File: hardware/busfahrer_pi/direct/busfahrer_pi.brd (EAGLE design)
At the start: 39.4 x 37.8 mm, 21 parts, among them Q1 20 MHz, X1 MKDSN1,5/2-5,08

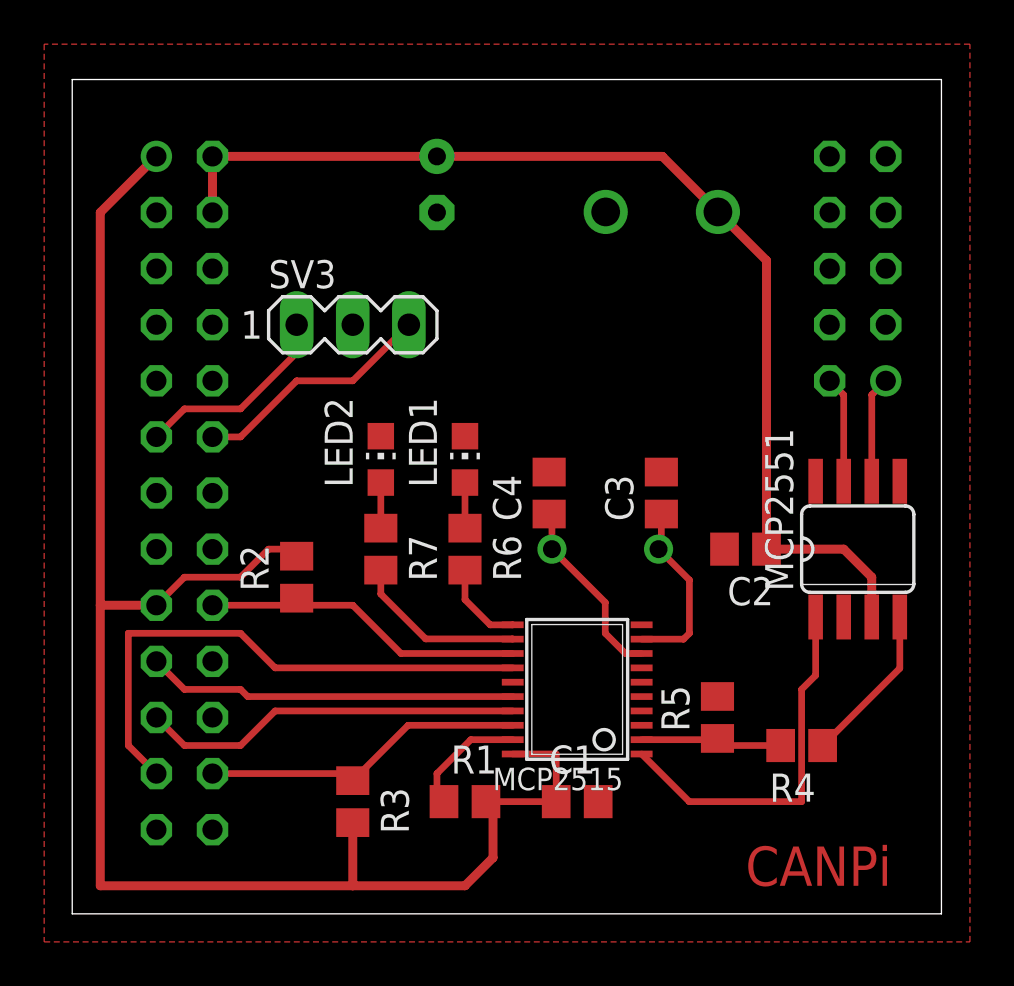
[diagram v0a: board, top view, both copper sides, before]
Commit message: some fixes
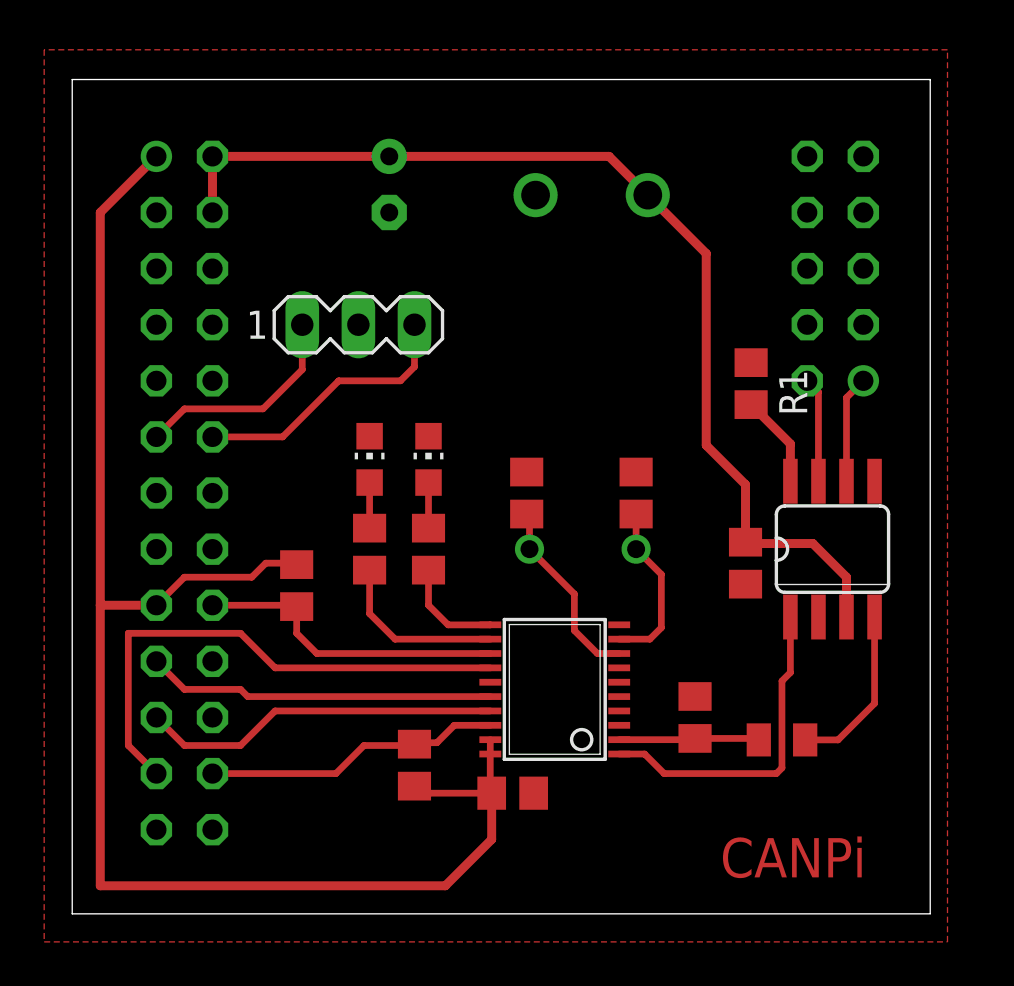
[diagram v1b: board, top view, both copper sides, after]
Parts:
- C3, C4: value 15p -> 22p
- R4: device rcl:R0805 -> rcl_patch:R0805
- R6, R7: value 220 -> 330
- moved R1 22.9 mm to (30.7, 24.0), turned to 270 degrees
- moved X1 3.27 mm to (23.5, 32.5)
- moved R3 3.25 mm to (15.5, 6.73)
- moved C1 2.95 mm to (19.9, 5.46)
- moved C5 2.16 mm to (14.4, 33.0)
- moved LED1 1.65 mm to (16.1, 20.6)
- moved R6 1.65 mm to (16.1, 16.5)
- moved C3 1.14 mm to (25.5, 19.1)
- moved MCP2551 1.14 mm to (34.4, 16.5)
- moved SV2 1.02 mm to (34.5, 29.2)
- moved R5 1.02 mm to (28.2, 8.89)
- moved C4 1.02 mm to (20.6, 19.1)
- moved MCP2515 1.02 mm to (21.8, 10.2)
- moved Q1 1.02 mm to (23.1, 16.5)
- moved R4 0.92 mm to (32.1, 7.87), turned to 0 degrees
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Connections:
- net N$5 renamed TXCAN
- removed net N$6: MCP2515.2, R4.2, R5.1
- removed net N$7: MCP2551.4, R4.1
- new net RXCAN: MCP2515.2, R4.1, R5.1
- new net RXCAN_5V: MCP2551.4, R4.2
- net +3V3: now also MCP2515.19; no longer R1.2
- net GND: now also R1.1; no longer MCP2551.8
- net N$1: now also MCP2551.8, R1.2; no longer MCP2515.19, R1.1
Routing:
- net RXCAN_5V: track 0.00 -> 7.74 mm
- net N$7: track 7.26 -> 0.00 mm
- net N$6: track 6.48 -> 0.00 mm
- net RXCAN: track 0.00 -> 6.40 mm
- net +3V3: track 75.3 -> 70.5 mm
- net +5V: track 49.7 -> 47.5 mm
- net TXCAN: track 16.8 -> 14.8 mm
- net POWER2: track 11.0 -> 12.4 mm
- net CS: track 14.8 -> 13.5 mm
- net N$1: track 5.47 -> 4.21 mm
- net SCK: track 24.9 -> 23.9 mm
- net MOSI: track 16.8 -> 15.8 mm
- net MISO: track 17.3 -> 16.3 mm
- net N$2: track 3.97 -> 4.76 mm
- net POWER1: track 9.20 -> 9.90 mm
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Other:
- board size 39.4 x 37.8 mm -> 38.8 x 37.8 mm
